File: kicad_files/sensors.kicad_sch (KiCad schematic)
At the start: 41 parts, among them J5 U.FL, U2 MS5611-01BA, U3 BMI088, U4 MMC5983MA, U5 MAX-M10S, U6 BMP388, U7 LSM6DSM

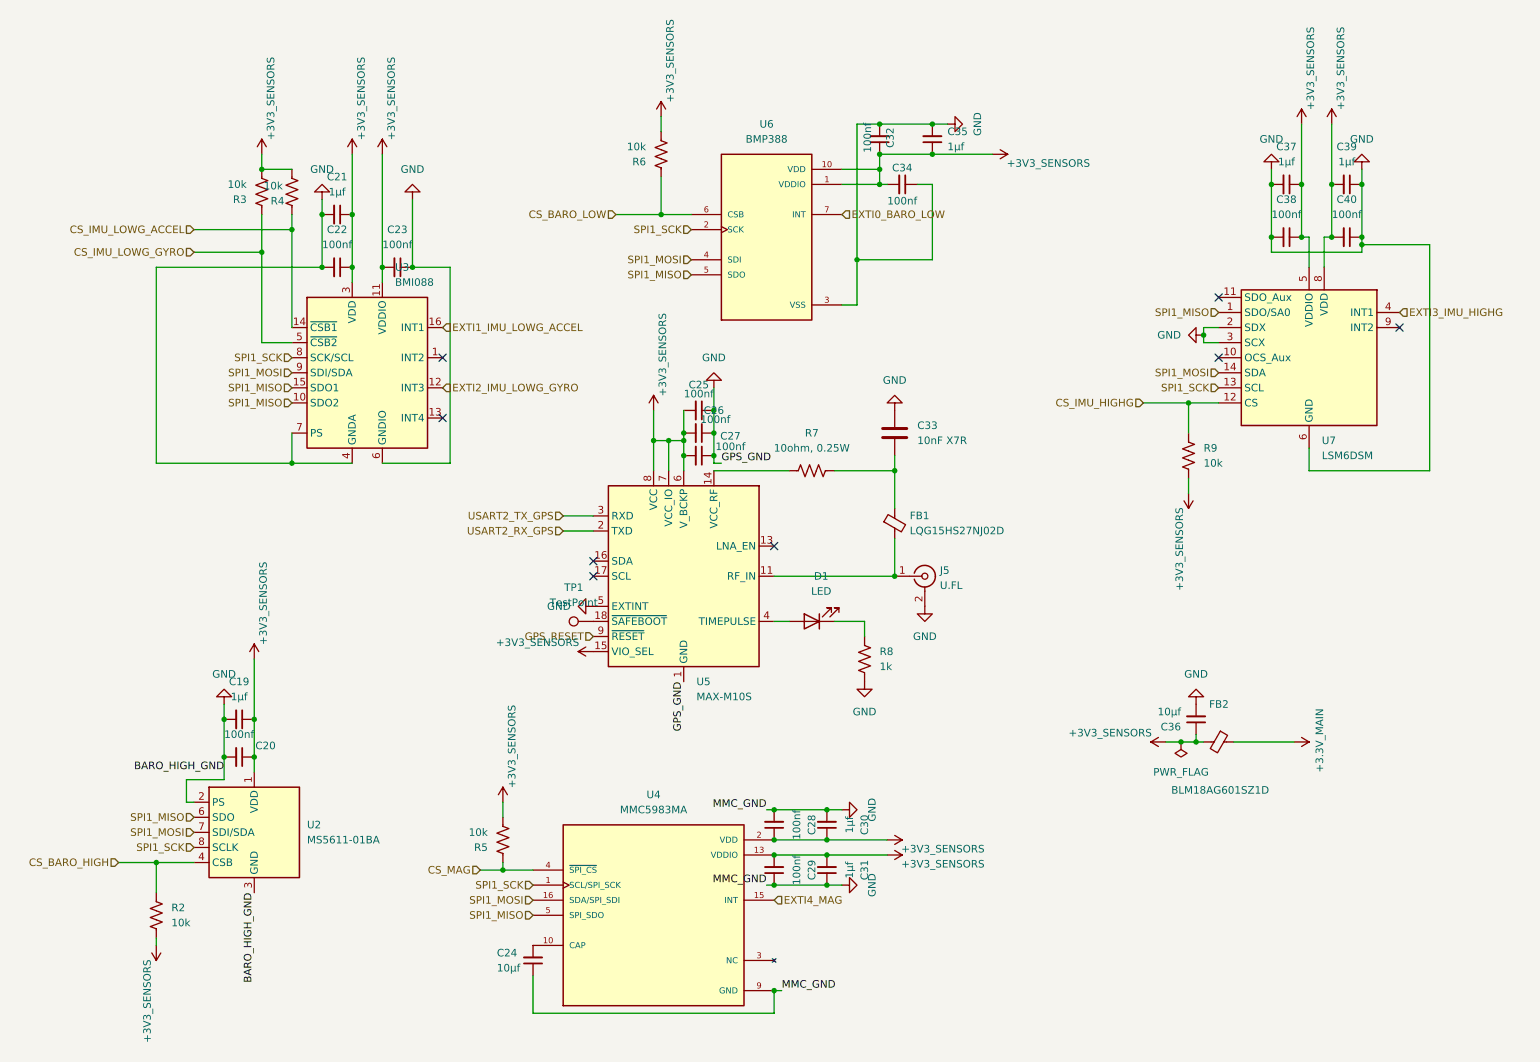
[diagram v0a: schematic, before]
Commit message: fix pyro adc
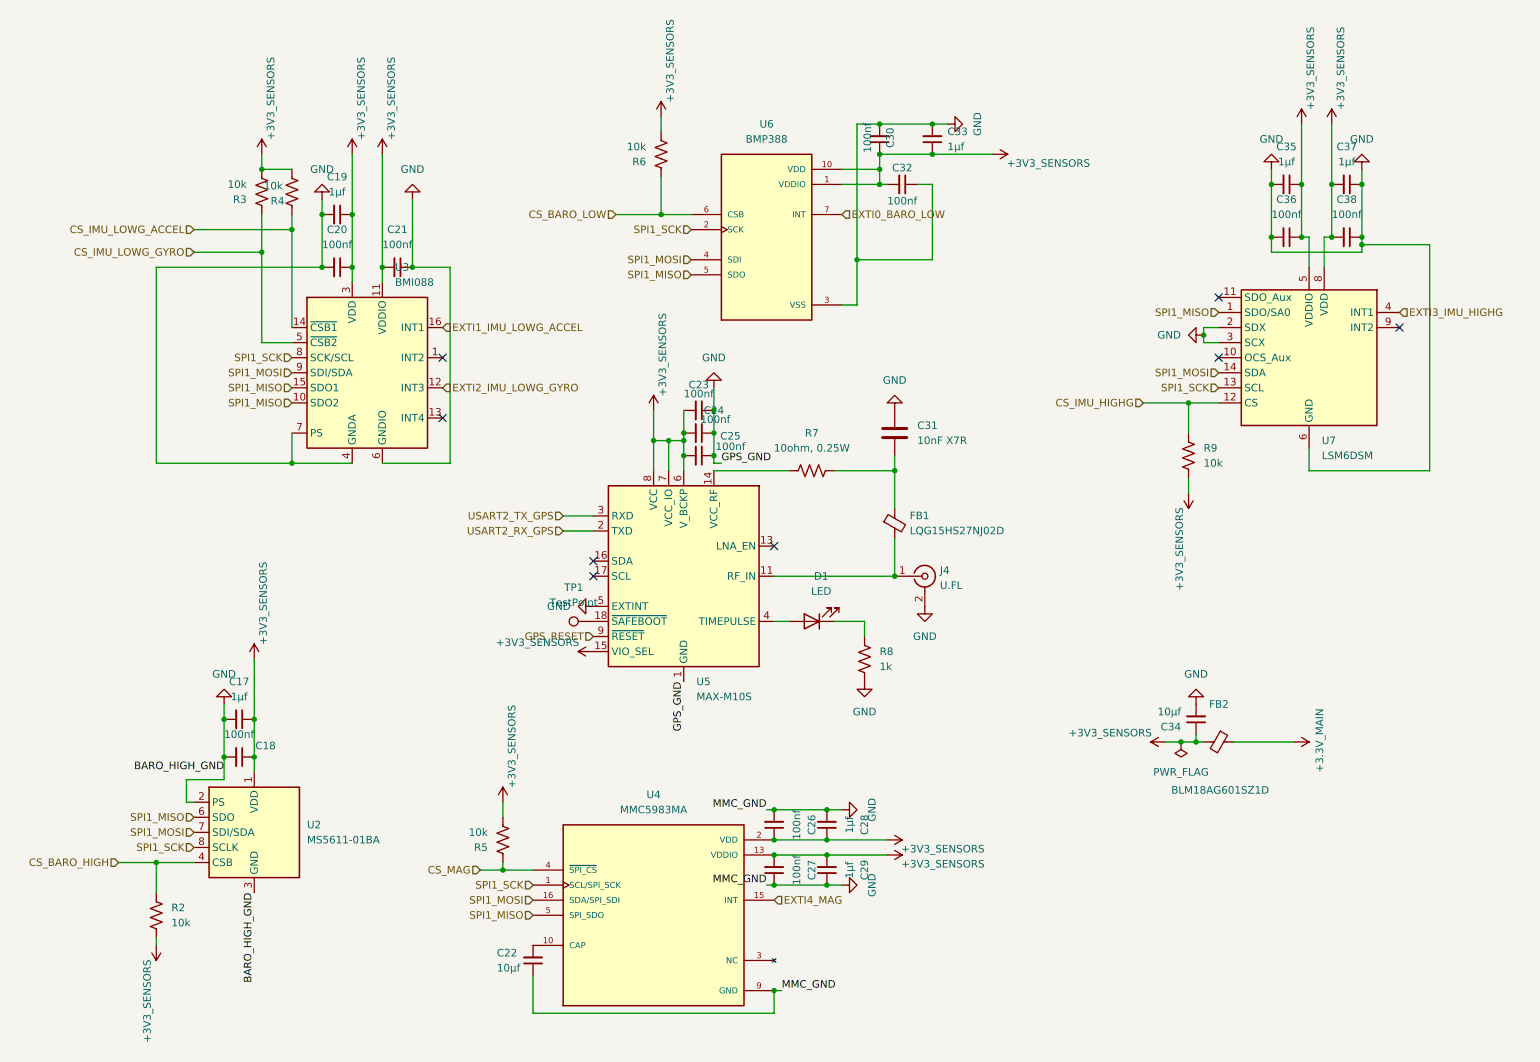
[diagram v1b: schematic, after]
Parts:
- renumbered C19 to C17, C20 to C18, C21 to C19, C22 to C20, C23 to C21, C24 to C22, C25 to C23, C26 to C24, C27 to C25, C28 to C26, C29 to C27, C30 to C28, C31 to C29, C32 to C30, C33 to C31, C34 to C32, C35 to C33, C36 to C34, C37 to C35, C38 to C36, C39 to C37, C40 to C38, J5 to J4
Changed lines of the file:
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@@
 		(dnp no)
 		(fields_autoplaced yes)
-		(property "Reference" "C38"
+		(property "Reference" "C36"
 			(at 241.2936 45.72 90)
 			(show_name no)
@@
 			(project "versorlite"
 				(path "/1a230af0-0a74-48f7-8607-b087121dda49/11200af7-3897-4179-b08c-df8c2996a93a"
-					(reference "C38")
+					(reference "C36")
 					(unit 1)
 				)
@@
 		(dnp no)
 		(fields_autoplaced yes)
-		(property "Reference" "J5"
+		(property "Reference" "J4"
 			(at 182.88 108.2431 0)
 			(show_name no)
@@
 			(project "versorlite"
 				(path "/1a230af0-0a74-48f7-8607-b087121dda49/11200af7-3897-4179-b08c-df8c2996a93a"
-					(reference "J5")
+					(reference "J4")
 					(unit 1)
 				)
@@
 		(dnp no)
 		(fields_autoplaced yes)
-		(property "Reference" "C33"
+		(property "Reference" "C31"
 			(at 179.07 83.8199 0)
 			(show_name no)
@@
 			(project "versorlite"
 				(path "/1a230af0-0a74-48f7-8607-b087121dda49/11200af7-3897-4179-b08c-df8c2996a93a"
-					(reference "C33")
+					(reference "C31")
 					(unit 1)
 				)
@@
 		(in_pos_files yes)
 		(dnp no)
-		(property "Reference" "C25"
+		(property "Reference" "C23"
 			(at 142.24 76.962 90)
 			(show_name no)
@@
 			(project "versorlite"
 				(path "/1a230af0-0a74-48f7-8607-b087121dda49/11200af7-3897-4179-b08c-df8c2996a93a"
-					(reference "C25")
+					(reference "C23")
 					(unit 1)
 				)
@@
 		(dnp no)
 		(fields_autoplaced yes)
-		(property "Reference" "C19"
+		(property "Reference" "C17"
 			(at 64.7636 127 90)
 			(show_name no)
@@
 			(project "versorlite"
 				(path "/1a230af0-0a74-48f7-8607-b087121dda49/11200af7-3897-4179-b08c-df8c2996a93a"
-					(reference "C19")
+					(reference "C17")
 					(unit 1)
 				)
@@
 		(in_pos_files yes)
 		(dnp no)
-		(property "Reference" "C27"
+		(property "Reference" "C25"
 			(at 147.574 85.598 90)
 			(show_name no)
@@
 			(project "versorlite"
 				(path "/1a230af0-0a74-48f7-8607-b087121dda49/11200af7-3897-4179-b08c-df8c2996a93a"
-					(reference "C27")
+					(reference "C25")
 					(unit 1)
 				)
@@
 		(dnp no)
 		(fields_autoplaced yes)
-		(property "Reference" "C36"
+		(property "Reference" "C34"
 			(at 223.52 134.6138 0)
 			(show_name no)
@@
 			(project "versorlite"
 				(path "/1a230af0-0a74-48f7-8607-b087121dda49/11200af7-3897-4179-b08c-df8c2996a93a"
-					(reference "C36")
+					(reference "C34")
 					(unit 1)
 				)
@@
 		(in_pos_files yes)
 		(dnp no)
-		(property "Reference" "C34"
+		(property "Reference" "C32"
 			(at 176.53 40.386 90)
 			(show_name no)
@@
 			(project "versorlite"
 				(path "/1a230af0-0a74-48f7-8607-b087121dda49/11200af7-3897-4179-b08c-df8c2996a93a"
-					(reference "C34")
+					(reference "C32")
 					(unit 1)
 				)
@@
 		(dnp no)
 		(fields_autoplaced yes)
-		(property "Reference" "C22"
+		(property "Reference" "C20"
 			(at 81.2736 50.8 90)
 			(show_name no)
@@
 			(project "versorlite"
 				(path "/1a230af0-0a74-48f7-8607-b087121dda49/11200af7-3897-4179-b08c-df8c2996a93a"
-					(reference "C22")
+					(reference "C20")
 					(unit 1)
 				)
@@
 		(dnp no)
 		(fields_autoplaced yes)
-		(property "Reference" "C23"
+		(property "Reference" "C21"
 			(at 91.4336 50.8 90)
 			(show_name no)
@@
 			(project "versorlite"
 				(path "/1a230af0-0a74-48f7-8607-b087121dda49/11200af7-3897-4179-b08c-df8c2996a93a"
-					(reference "C23")
+					(reference "C21")
 					(unit 1)
 				)
@@
 		(dnp no)
 		(fields_autoplaced yes)
-		(property "Reference" "C40"
+		(property "Reference" "C38"
 			(at 251.4536 45.72 90)
 			(show_name no)
@@
 			(project "versorlite"
 				(path "/1a230af0-0a74-48f7-8607-b087121dda49/11200af7-3897-4179-b08c-df8c2996a93a"
-					(reference "C40")
+					(reference "C38")
 					(unit 1)
 				)
@@
 		(in_pos_files yes)
 		(dnp no)
-		(property "Reference" "C24"
+		(property "Reference" "C22"
 			(at 108.204 172.72 0)
 			(show_name no)
@@
 			(project "versorlite"
 				(path "/1a230af0-0a74-48f7-8607-b087121dda49/11200af7-3897-4179-b08c-df8c2996a93a"
-					(reference "C24")
+					(reference "C22")
 					(unit 1)
 				)
@@
 		(in_pos_files yes)
 		(dnp no)
-		(property "Reference" "C32"
+		(property "Reference" "C30"
 			(at 174.498 35.306 90)
 			(show_name no)
@@
 			(project "versorlite"
 				(path "/1a230af0-0a74-48f7-8607-b087121dda49/11200af7-3897-4179-b08c-df8c2996a93a"
-					(reference "C32")
+					(reference "C30")
 					(unit 1)
 				)
@@
 		(dnp no)
 		(fields_autoplaced yes)
-		(property "Reference" "C35"
+		(property "Reference" "C33"
 			(at 184.15 34.2835 0)
 			(show_name no)
@@
 			(project "versorlite"
 				(path "/1a230af0-0a74-48f7-8607-b087121dda49/11200af7-3897-4179-b08c-df8c2996a93a"
-					(reference "C35")
+					(reference "C33")
 					(unit 1)
 				)
@@
 		(dnp no)
 		(fields_autoplaced yes)
-		(property "Reference" "C21"
+		(property "Reference" "C19"
 			(at 81.2736 41.91 90)
 			(show_name no)
@@
 			(project "versorlite"
 				(path "/1a230af0-0a74-48f7-8607-b087121dda49/11200af7-3897-4179-b08c-df8c2996a93a"
-					(reference "C21")
+					(reference "C19")
 					(unit 1)
 				)
@@
 		(dnp no)
 		(fields_autoplaced yes)
-		(property "Reference" "C31"
+		(property "Reference" "C29"
 			(at 170.18 158.7436 90)
 			(show_name no)
@@
 			(project "versorlite"
 				(path "/1a230af0-0a74-48f7-8607-b087121dda49/11200af7-3897-4179-b08c-df8c2996a93a"
-					(reference "C31")
+					(reference "C29")
 					(unit 1)
 				)
@@
 		(dnp no)
 		(fields_autoplaced yes)
-		(property "Reference" "C39"
+		(property "Reference" "C37"
 			(at 251.4536 36.83 90)
 			(show_name no)
@@
 			(project "versorlite"
 				(path "/1a230af0-0a74-48f7-8607-b087121dda49/11200af7-3897-4179-b08c-df8c2996a93a"
-					(reference "C39")
+					(reference "C37")
 					(unit 1)
 				)
@@
 		(dnp no)
 		(fields_autoplaced yes)
-		(property "Reference" "C28"
+		(property "Reference" "C26"
 			(at 161.29 151.1236 90)
 			(show_name no)
@@
 			(project "versorlite"
 				(path "/1a230af0-0a74-48f7-8607-b087121dda49/11200af7-3897-4179-b08c-df8c2996a93a"
-					(reference "C28")
+					(reference "C26")
 					(unit 1)
 				)
@@
 		(dnp no)
 		(fields_autoplaced yes)
-		(property "Reference" "C29"
+		(property "Reference" "C27"
 			(at 161.29 158.7436 90)
 			(show_name no)
@@
 			(project "versorlite"
 				(path "/1a230af0-0a74-48f7-8607-b087121dda49/11200af7-3897-4179-b08c-df8c2996a93a"
-					(reference "C29")
+					(reference "C27")
 					(unit 1)
 				)
@@
 		(in_pos_files yes)
 		(dnp no)
-		(property "Reference" "C26"
+		(property "Reference" "C24"
 			(at 144.78 81.28 90)
 			(show_name no)
@@
 			(project "versorlite"
 				(path "/1a230af0-0a74-48f7-8607-b087121dda49/11200af7-3897-4179-b08c-df8c2996a93a"
-					(reference "C26")
+					(reference "C24")
 					(unit 1)
 				)
@@
 		(dnp no)
 		(fields_autoplaced yes)
-		(property "Reference" "C37"
+		(property "Reference" "C35"
 			(at 241.2936 36.83 90)
 			(show_name no)
@@
 			(project "versorlite"
 				(path "/1a230af0-0a74-48f7-8607-b087121dda49/11200af7-3897-4179-b08c-df8c2996a93a"
-					(reference "C37")
+					(reference "C35")
 					(unit 1)
 				)
@@
 		(in_pos_files yes)
 		(dnp no)
-		(property "Reference" "C20"
+		(property "Reference" "C18"
 			(at 69.215 137.795 90)
 			(show_name no)
@@
 			(project "versorlite"
 				(path "/1a230af0-0a74-48f7-8607-b087121dda49/11200af7-3897-4179-b08c-df8c2996a93a"
-					(reference "C20")
+					(reference "C18")
 					(unit 1)
 				)
@@
 		(dnp no)
 		(fields_autoplaced yes)
-		(property "Reference" "C30"
+		(property "Reference" "C28"
 			(at 170.18 151.1236 90)
 			(show_name no)
@@
 			(project "versorlite"
 				(path "/1a230af0-0a74-48f7-8607-b087121dda49/11200af7-3897-4179-b08c-df8c2996a93a"
-					(reference "C30")
+					(reference "C28")
 					(unit 1)
 				)
